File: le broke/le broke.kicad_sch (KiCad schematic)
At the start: 37 parts, among them U1 ProMicro

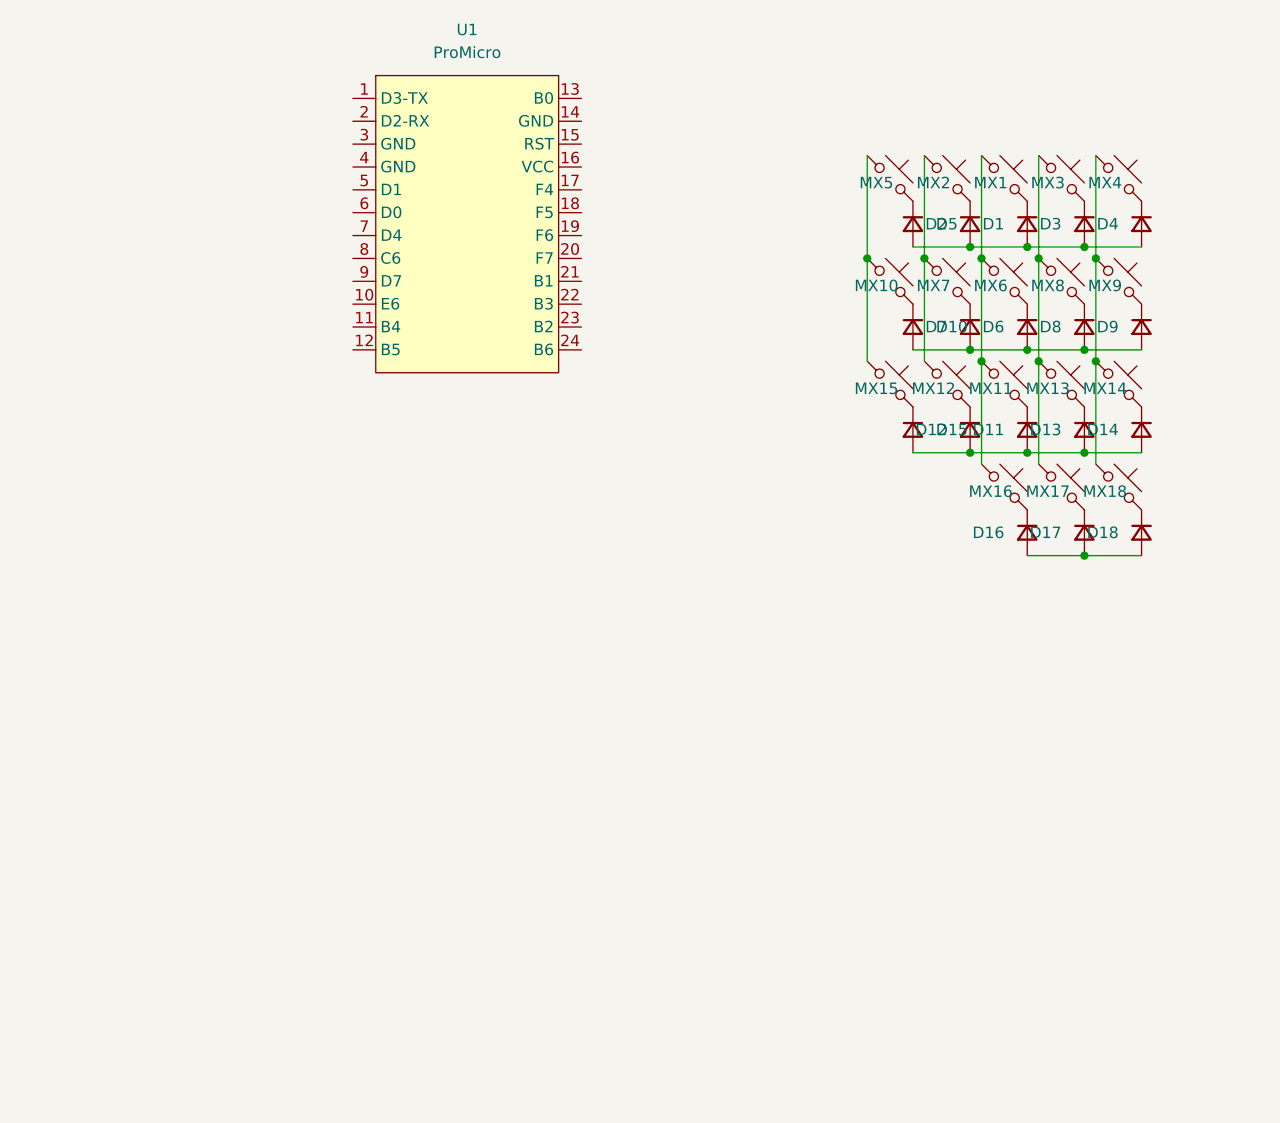
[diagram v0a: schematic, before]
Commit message: a
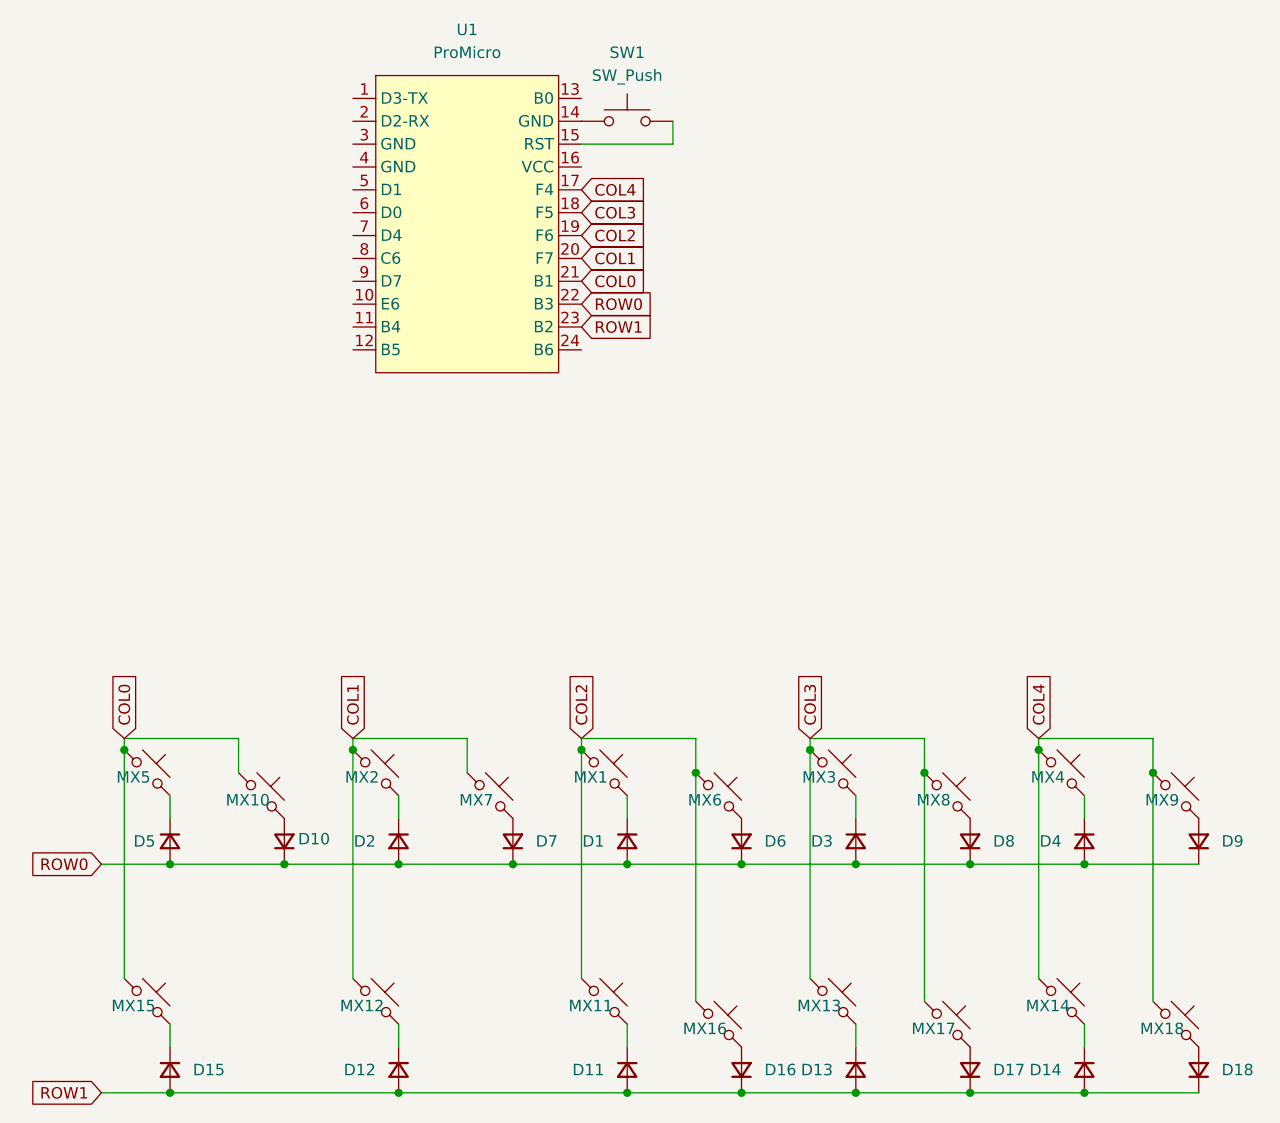
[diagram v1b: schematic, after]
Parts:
- added SW1: SW_Push, Button_Switch_THT:SW_PUSH_6mm, symbol Switch:SW_Push
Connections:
- net COL0: now reaches MX10.1, MX15.1, MX5.1
- net COL0: now also U1.21 (B1)
- net COL3: now reaches MX13.1, MX17.1, MX3.1, MX8.1
- net COL3: now also U1.18 (F5)
- net at MX7.2: now also D7.2 (A); no longer D7.1 (K)
- net COL4: now reaches MX14.1, MX18.1, MX4.1, MX9.1
- net COL4: now also U1.17 (F4)
- net COL2: now reaches MX1.1, MX11.1, MX16.1, MX6.1
- net COL2: now also U1.19 (F6)
- net ROW1: now reaches D11.2 (A), D12.2 (A), D13.2 (A), D14.2 (A), D15.2 (A)
- net ROW1: now also D16.1 (K), D17.1 (K), D18.1 (K), U1.23 (B2)
- net at U1.14 (GND): now also SW1.1
- net at U1.15 (RST): now also SW1.2
- net COL1: now reaches U1.20 (F7)
- net COL1: now also MX12.1, MX2.1, MX7.1
- net ROW0: now reaches U1.22 (B3)
- net ROW0: now also D1.2 (A), D10.1 (K), D2.2 (A), D3.2 (A), D4.2 (A), D5.2 (A), D6.1 (K), D7.1 (K), D8.1 (K), D9.1 (K)
- net at MX8.2: now also D8.2 (A); no longer D8.1 (K)
- net at MX9.2: now also D9.2 (A); no longer D9.1 (K)
- net at MX6.2: now also D6.2 (A); no longer D6.1 (K)
- net at MX10.2: now also D10.2 (A); no longer D10.1 (K)
- net at MX18.2: now also D18.2 (A); no longer D18.1 (K)
- net at MX17.2: now also D17.2 (A); no longer D17.1 (K)
- net at MX16.2: now also D16.2 (A); no longer D16.1 (K)
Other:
- moved on the sheet: D1, D10, D11, D12, D13, D14, D15, D16, D17, D18, D2, D3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
